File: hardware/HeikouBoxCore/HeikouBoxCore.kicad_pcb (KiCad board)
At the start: 2 copper layers, 40 x 40 mm, 35 parts, among them J1 L, J2 B, J3 R, J4 T, U1 EP3C25E144

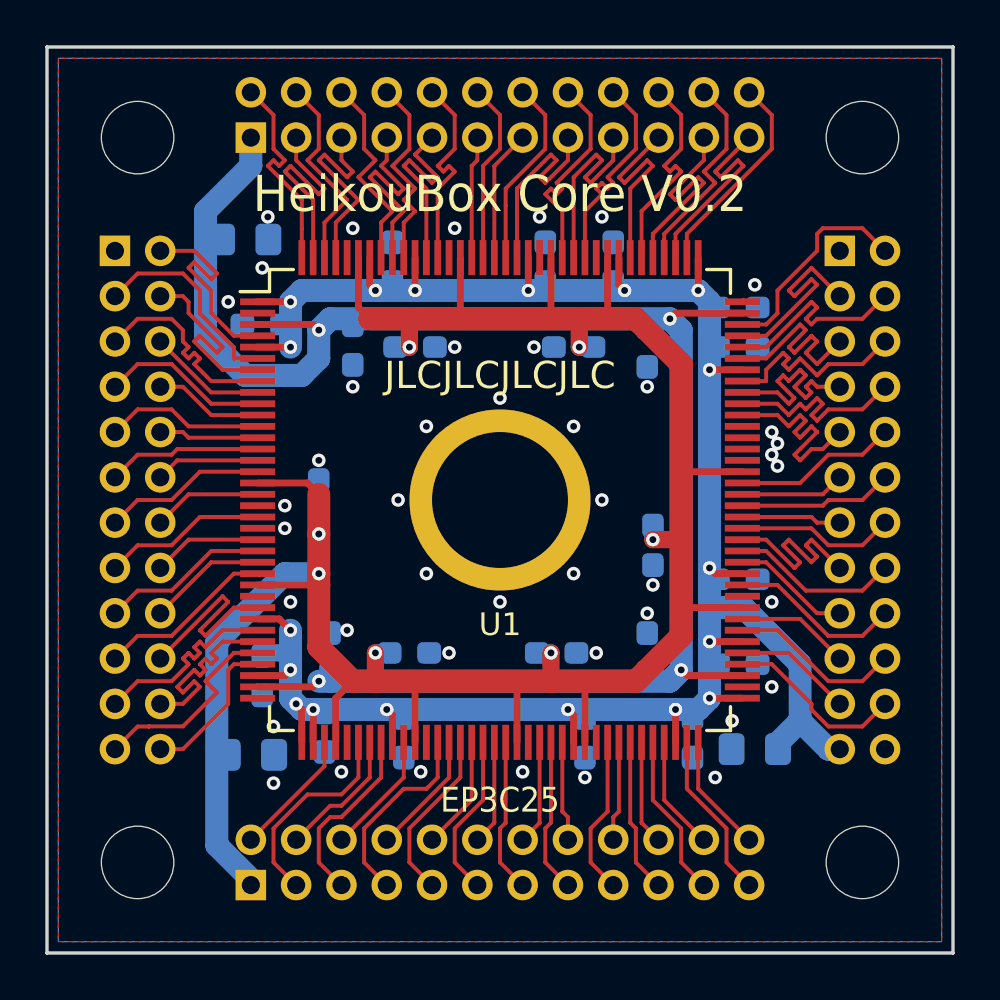
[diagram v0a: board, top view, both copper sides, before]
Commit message: Core: Update gerbers to V0.2
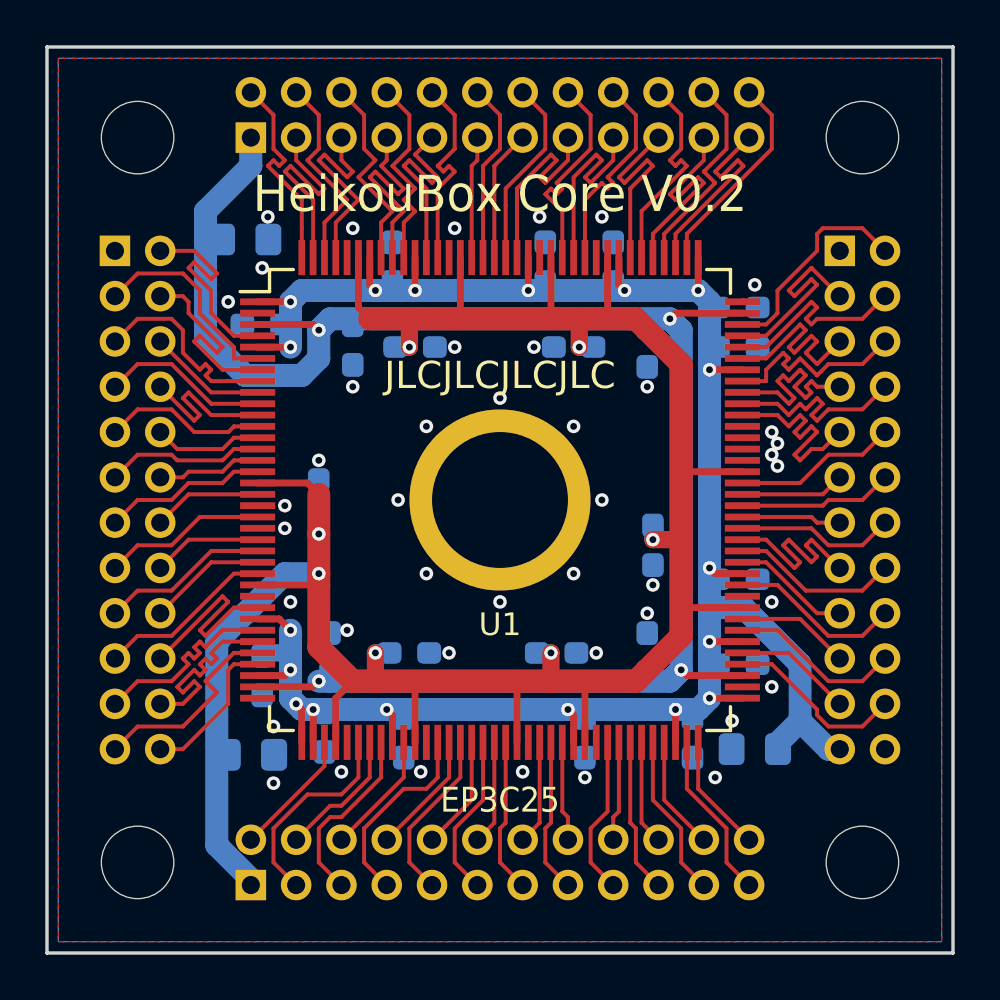
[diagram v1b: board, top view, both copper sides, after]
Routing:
- net /SIGMA1: track 4.82 -> 7.35 mm
- net /TDI: track 4.61 -> 5.41 mm
